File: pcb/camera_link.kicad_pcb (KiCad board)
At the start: 2 copper layers, 159.3 x 14.5 mm, 12 parts, among them J1 RJ45_pyControl, J2 Screw_Terminal_01x08

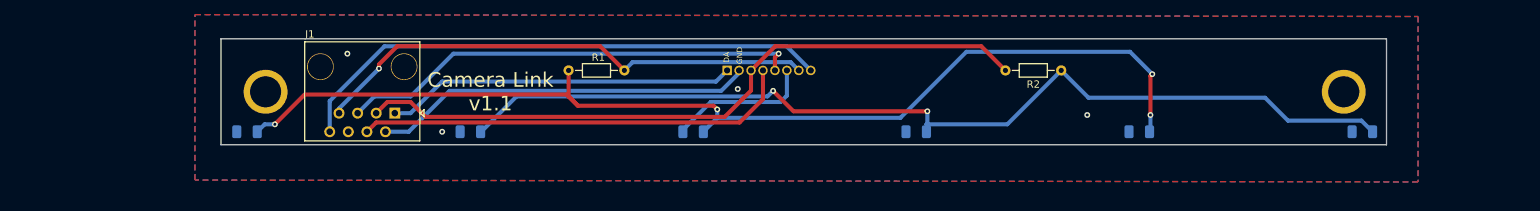
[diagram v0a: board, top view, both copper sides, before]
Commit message: pcbv1.2
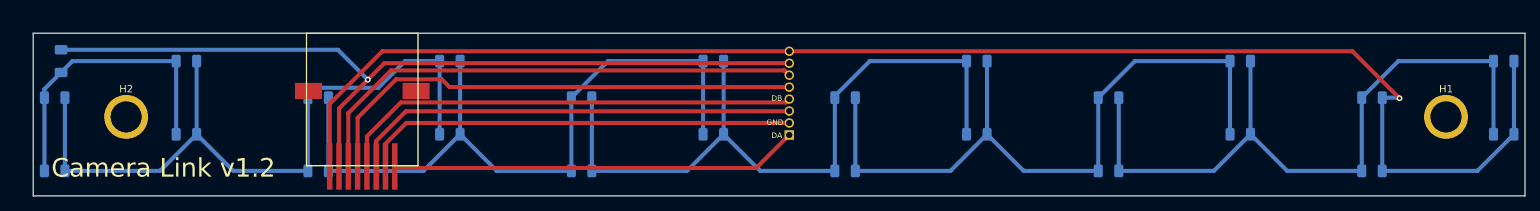
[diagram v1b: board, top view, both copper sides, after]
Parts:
- removed R2: R_US, Resistor_THT:R_Axial_DIN0204_L3.6mm_D1.6mm_P7.62mm_Horizontal
- added D10: LED, LED_SMD:LED_1206_3216Metric, B.Cu at (157.9, 113.0)
- added D11: LED, LED_SMD:LED_1206_3216Metric, B.Cu at (175.9, 118.0)
- added D12: LED, LED_SMD:LED_1206_3216Metric, B.Cu at (157.9, 123.0)
- added D13: LED, LED_SMD:LED_1206_3216Metric, B.Cu at (139.9, 108.0)
- added D14: LED, LED_SMD:LED_1206_3216Metric, B.Cu at (121.9, 113.0)
- added D15: LED, LED_SMD:LED_1206_3216Metric, B.Cu at (139.9, 118.0)
- added D16: LED, LED_SMD:LED_1206_3216Metric, B.Cu at (121.9, 123.0)
- added D17: LED, LED_SMD:LED_1206_3216Metric, B.Cu at (103.9, 108.0)
- added D18: LED, LED_SMD:LED_1206_3216Metric, B.Cu at (85.9, 113.0)
- added D19: LED, LED_SMD:LED_1206_3216Metric, B.Cu at (103.9, 118.0)
- added D20: LED, LED_SMD:LED_1206_3216Metric, B.Cu at (85.9, 123.0)
- added D21: LED, LED_SMD:LED_1206_3216Metric, B.Cu at (67.9, 108.0)
- added D22: LED, LED_SMD:LED_1206_3216Metric, B.Cu at (49.9, 113.0)
- added D23: LED, LED_SMD:LED_1206_3216Metric, B.Cu at (67.9, 118.0)
- added D24: LED, LED_SMD:LED_1206_3216Metric, B.Cu at (49.9, 123.0)
- added D7: LED, LED_SMD:LED_1206_3216Metric, B.Cu at (211.9, 118.0)
- added D8: LED, LED_SMD:LED_1206_3216Metric, B.Cu at (193.9, 123.0)
- added D9: LED, LED_SMD:LED_1206_3216Metric, B.Cu at (175.9, 108.0)
- J1: footprint asl_footprints:RJ45_THP_Vertical -> asl_footprints:RJ45_SMD
- R1: value R_US -> 9Ω; footprint Resistor_THT:R_Axial_DIN0204_L3.6mm_D1.6mm_P7.62mm_Horizontal -> Resistor_SMD:R_1206_3216Metric_Pad1.30x1.75mm_HandSolder; moved to B.Cu
- moved D1 172.0 mm to (247.9, 108.0), turned to 0 degrees
- moved D4 123.3 mm to (229.9, 123.0), turned to 0 degrees
- moved D2 92.9 mm to (229.9, 112.9), turned to 0 degrees
- moved R1 77.0 mm to (50.8, 108.0), turned to 90 degrees
- moved D3 49.8 mm to (247.9, 118.0), turned to 0 degrees
- moved D5 45.3 mm to (211.9, 108.0), turned to 0 degrees
- moved D6 35.0 mm to (193.9, 113.0), turned to 0 degrees
- moved H2 19.4 mm to (59.7, 115.6)
- moved H1 14.4 mm to (240.0, 115.6)
- moved J1 4.57 mm to (91.9, 104.1)
- moved J2 4.16 mm to (150.3, 112.3), turned to 180 degrees
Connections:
- net Net-(J1-Pad2) renamed /GND
- D1 pad 2: /5VDC -> Net-(D1-Pad2)
- D2 pad 2: /5VDC -> Net-(D1-Pad2)
- D3 pad 2: /5VDC -> Net-(D1-Pad2)
- D4 pad 1: Net-(D4-Pad1) -> Net-(D1-Pad1)
- D4 pad 2: /5VDC -> Net-(D1-Pad2)
- D5 pad 1: Net-(D4-Pad1) -> Net-(D10-Pad2)
- D5 pad 2: /5VDC -> Net-(D1-Pad1)
- D6 pad 1: Net-(D4-Pad1) -> Net-(D10-Pad2)
- D6 pad 2: /5VDC -> Net-(D1-Pad1)
- J1 pad 6: /5VDC -> Net-(J1-Pad6)
- J1 pad 8: Net-(J1-Pad8) -> Net-(D1-Pad2)
- J2 pad 6: /5VDC -> Net-(J1-Pad6)
- J2 pad 8: Net-(J1-Pad8) -> Net-(D1-Pad2)
- R1 pad 1: Net-(J1-Pad7) -> Net-(D21-Pad1)
- R1 pad 2: Net-(D1-Pad1) -> Net-(J1-Pad7)
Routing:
- net Net-(D1-Pad2): track 0.00 -> 202.8 mm, vias 0 -> 1
- net Net-(D4-Pad1): track 133.7 -> 0.00 mm, vias 2 -> 0
- net Net-(D10-Pad1): track 0.00 -> 97.8 mm
- net Net-(D13-Pad1): track 0.00 -> 97.4 mm
- net Net-(D10-Pad2): track 0.00 -> 97.4 mm
- net Net-(D17-Pad1): track 0.00 -> 97.4 mm
- net Net-(J1-Pad8): track 74.4 -> 0.00 mm
- net Net-(J1-Pad6): track 0.00 -> 70.2 mm
- net Net-(D1-Pad1): track 147.5 -> 97.4 mm, vias 4 -> 0
- net Net-(J1-Pad7): track 69.6 -> 115.6 mm
- net Net-(D21-Pad1): track 0.00 -> 40.8 mm
- net Net-(J1-Pad3): track 94.8 -> 61.6 mm
- net /5VDC: track 19.6 -> 0.00 mm, vias 4 -> 0
- net Net-(J1-Pad1): track 47.8 -> 55.9 mm
- net /GND: track 52.0 -> 59.4 mm
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- removed copper zone on B.Cu, net /5VDC
- removed copper zone on F.Cu, net /5VDC
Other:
- board size 159.3 x 14.5 mm -> 203.8 x 22.2 mm
- board text added: "Camera Link v1.2"
- board text added: "DB"
- board text removed: "Camera Link v1.1"
